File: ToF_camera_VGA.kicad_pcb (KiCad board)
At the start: 4 copper layers, 159.9 x 99.9 mm, 51 parts, among them J1 Conn_01x22, J2 Conn_01x08, J8 Conn_01x02, SW1 SW_Push, U1 TPS82150, U2 MLX75027, U3 TPS82150, U4 TPS82150, U5 TPSM84624, U6 PCA9306, Y1 Crystal

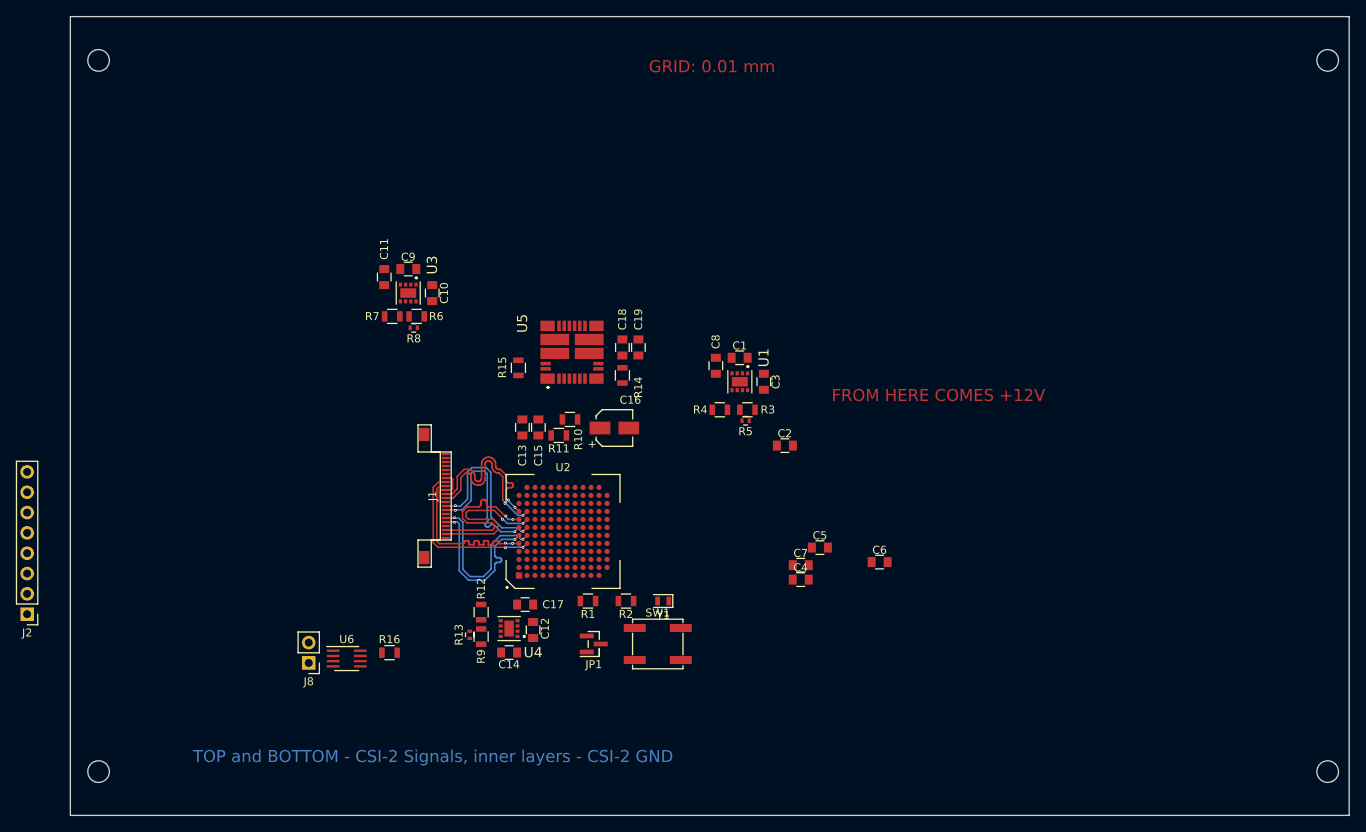
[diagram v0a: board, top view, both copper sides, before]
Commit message: Almost there... minor modifications for production needed
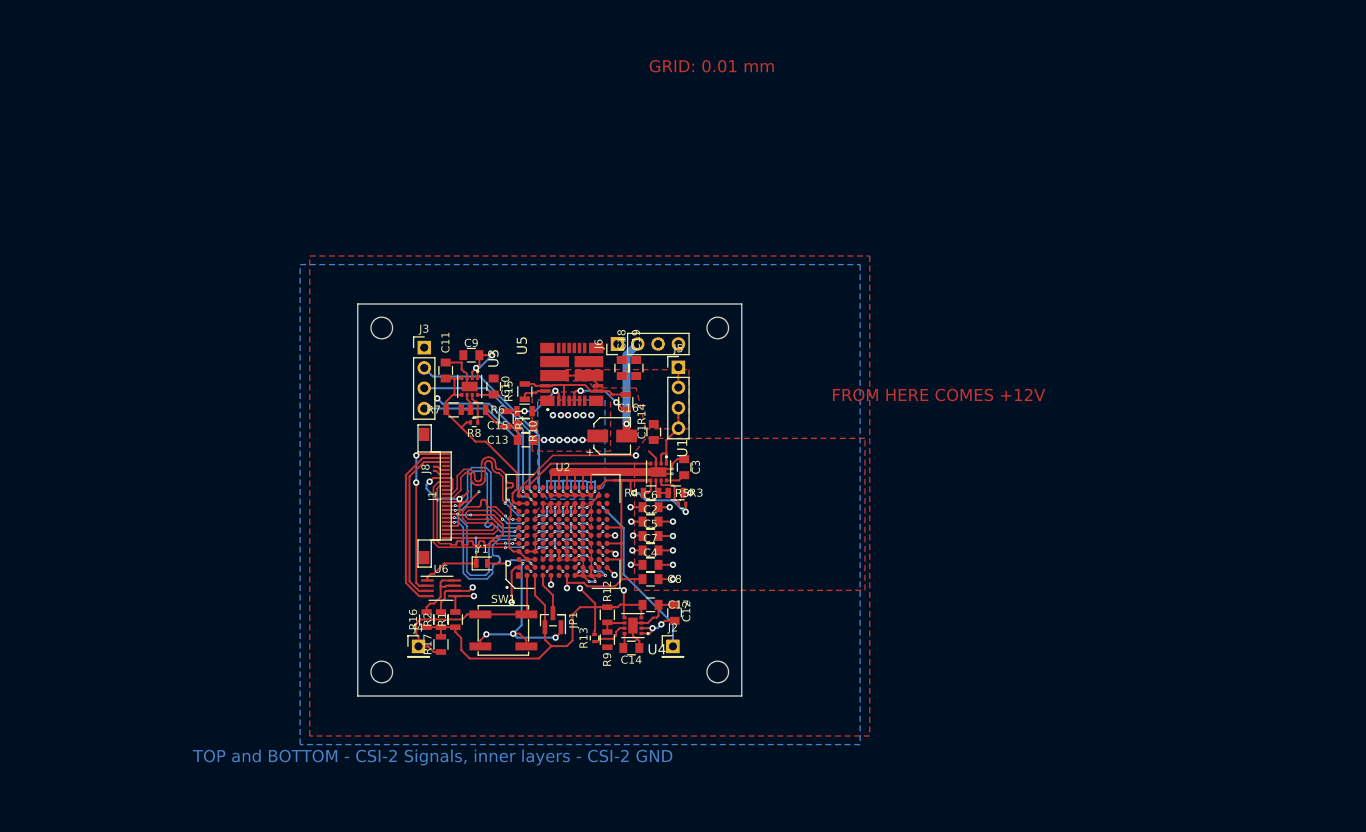
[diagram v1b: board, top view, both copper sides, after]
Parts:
- added J3: Conn_01x04, Pin_Headers:Pin_Header_Straight_1x04_Pitch2.54mm, F.Cu at (99.3, 86.5)
- added J4: Conn_01x01, Pin_Headers:Pin_Header_Straight_1x01_Pitch2.54mm, F.Cu at (98.6, 123.8)
- added J5: Conn_01x04, Pin_Headers:Pin_Header_Straight_1x04_Pitch2.54mm, F.Cu at (131.1, 88.9)
- added J6: Conn_01x04, Pin_Headers:Pin_Header_Straight_1x04_Pitch2.54mm, F.Cu at (123.5, 86.0)
- added R17: R, Resistors_SMD:R_0805, F.Cu at (101.4, 123.5)
- J2: value Conn_01x08 -> Conn_01x01; footprint Pin_Headers:Pin_Header_Straight_1x08_Pitch2.54mm -> Pin_Headers:Pin_Header_Straight_1x01_Pitch2.54mm
- J8: footprint Pin_Headers:Pin_Header_Straight_1x02_Pitch2.54mm -> Resistors_SMD:R_0201_NoSilk
- moved MK2 83.3 mm to (136.0, 84.0)
- moved J2 80.8 mm to (130.4, 123.8), turned to 0 degrees
- moved MK4 77.2 mm to (136.0, 127.0)
- moved MK1 48.7 mm to (94.0, 84.0)
- moved MK3 37.5 mm to (94.0, 127.0)
- moved C6 29.4 mm to (127.6, 106.4)
- moved J8 28.9 mm to (100.6, 101.6), turned to 90 degrees
- moved C8 27.9 mm to (127.6, 115.4), turned to 0 degrees
- moved R2 23.2 mm to (101.4, 120.5), turned to 90 degrees
- moved Y1 23.2 mm to (106.5, 113.4), turned to 0 degrees
- moved C5 21.2 mm to (127.6, 110.0)
- moved SW1 19.4 mm to (109.2, 121.8)
- moved C2 19.3 mm to (127.6, 108.2)
- moved C4 18.9 mm to (127.6, 113.6)
- moved C7 18.9 mm to (127.6, 111.8)
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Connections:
- R1 pad 2: Net-(J2-Pad6) -> Net-(R1-Pad2)
- R13 pad 1: /PGOOD_VDD -> /PGOOD_1.8V
- R2 pad 2: Net-(J2-Pad7) -> Net-(R2-Pad2)
- R5 pad 1: /PGOOD_VDD -> /PGOOD_VDDA
- SW1 pad 1: Net-(J2-Pad2) -> Net-(J4-Pad1)
- U1 pad 7: /PGOOD_VDD -> /PGOOD_VDDA
- U2 pad A2: Net-(J2-Pad2) -> Net-(J4-Pad1)
- U2 pad A5: Net-(J2-Pad6) -> Net-(R1-Pad2)
- U2 pad B5: Net-(J2-Pad7) -> Net-(R2-Pad2)
- U2 pad K11: Net-(J2-Pad8) -> Net-(J2-Pad1)
- U2 pad K3: Net-(J2-Pad5) -> Net-(J3-Pad4)
- U2 pad L2: Net-(J2-Pad1) -> Net-(J3-Pad1)
- U2 pad L3: Net-(J2-Pad4) -> Net-(J3-Pad3)
- U2 pad L4: Net-(J2-Pad3) -> Net-(J3-Pad2)
- U4 pad 7: /PGOOD_VDD -> /PGOOD_1.8V
- U6 pad 5: Net-(J2-Pad6) -> Net-(R1-Pad2)
- U6 pad 6: Net-(J2-Pad7) -> Net-(R2-Pad2)
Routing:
- net GNDD: track 6.02 -> 192.0 mm, vias 0 -> 65
- net GNDA: track 0.00 -> 103.9 mm, vias 0 -> 14
- net +1V8: track 0.00 -> 100.7 mm, vias 0 -> 5
- net VDDA: track 0.00 -> 77.0 mm, vias 0 -> 4
- net VDD: track 0.00 -> 36.6 mm
- net +1V2: track 0.00 -> 36.4 mm, vias 0 -> 19
- net +12V: track 0.00 -> 34.1 mm, vias 0 -> 4
- net Net-(J3-Pad1): track 0.00 -> 29.0 mm, vias 0 -> 2
- net Net-(J3-Pad2): track 0.00 -> 25.5 mm, vias 0 -> 1
- net Net-(J4-Pad1): track 0.00 -> 25.2 mm
- net Net-(J3-Pad3): track 0.00 -> 23.7 mm, vias 0 -> 1
- net /SDA_Pi: track 0.00 -> 22.7 mm
- net Net-(J3-Pad4): track 0.00 -> 22.6 mm, vias 0 -> 1
- net Net-(J2-Pad1): track 0.00 -> 21.7 mm, vias 0 -> 1
- net /3V3_Pi: track 0.00 -> 21.2 mm, vias 0 -> 2
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- added copper zone on F.Cu, net +12V
- added copper zone on In2.Cu, net +12V
- added copper zone on B.Cu, net +1V2
- added copper zone on F.Cu, net +1V2
- added copper zone on In1.Cu, net +1V2
- added copper zone on In2.Cu, net +1V2
- added copper zone on F.Cu, net GNDA
- added copper zone on In1.Cu, net GNDA
- added copper zone on B.Cu, net GNDD
- added copper zone on F.Cu, net GNDD
- added copper zone on In1.Cu, net GNDD
- added copper zone on In2.Cu, net GNDD
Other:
- board size 159.9 x 99.9 mm -> 48 x 49 mm
